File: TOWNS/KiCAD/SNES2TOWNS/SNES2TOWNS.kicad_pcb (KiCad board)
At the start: 2 copper layers, 64.8 x 50.8 mm, 16 parts, among them J1 DE9_Receptacle, J6 SNES_CONTROLLER, J8 ArduinoNANOP1_P15, J9 ArduinoNANOP16_P30, SW1 PCM13SMTR, U1 74HC157, U2 74HC157

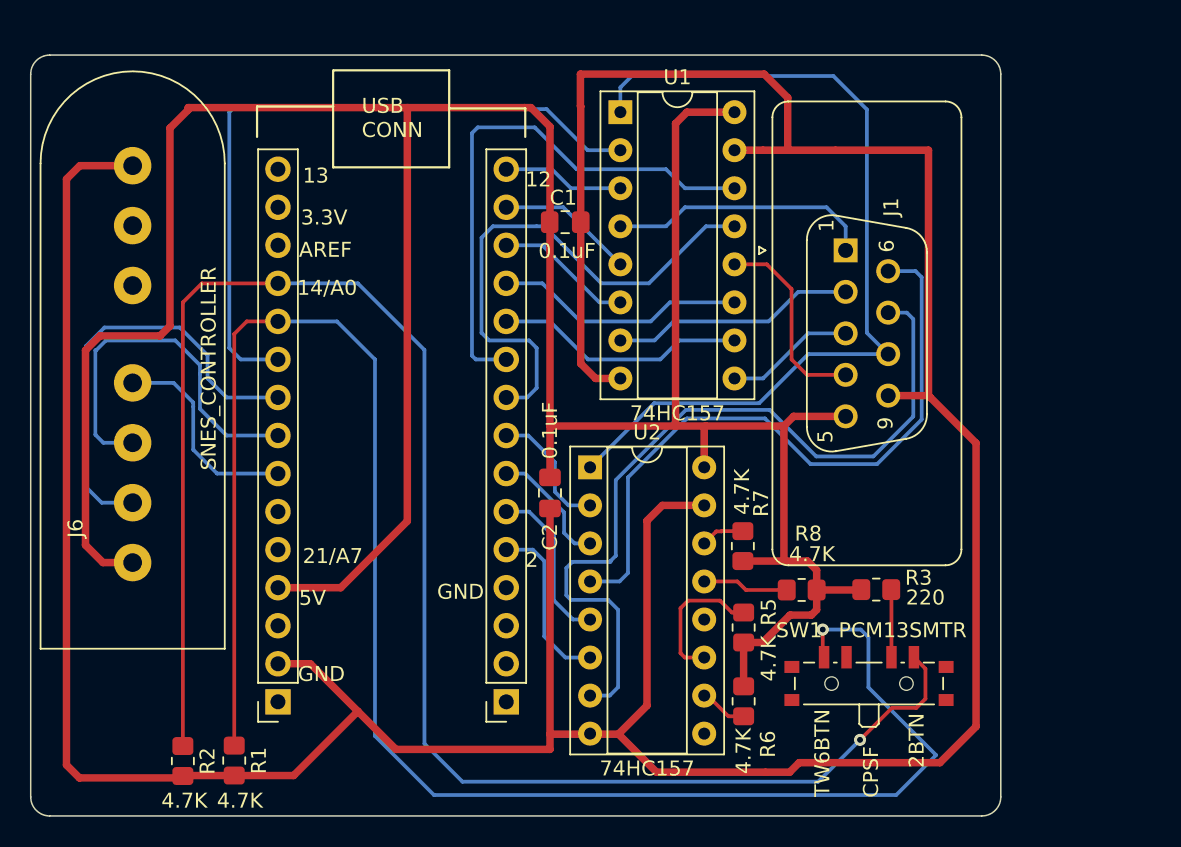
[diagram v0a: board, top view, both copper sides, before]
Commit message: Updating PCB
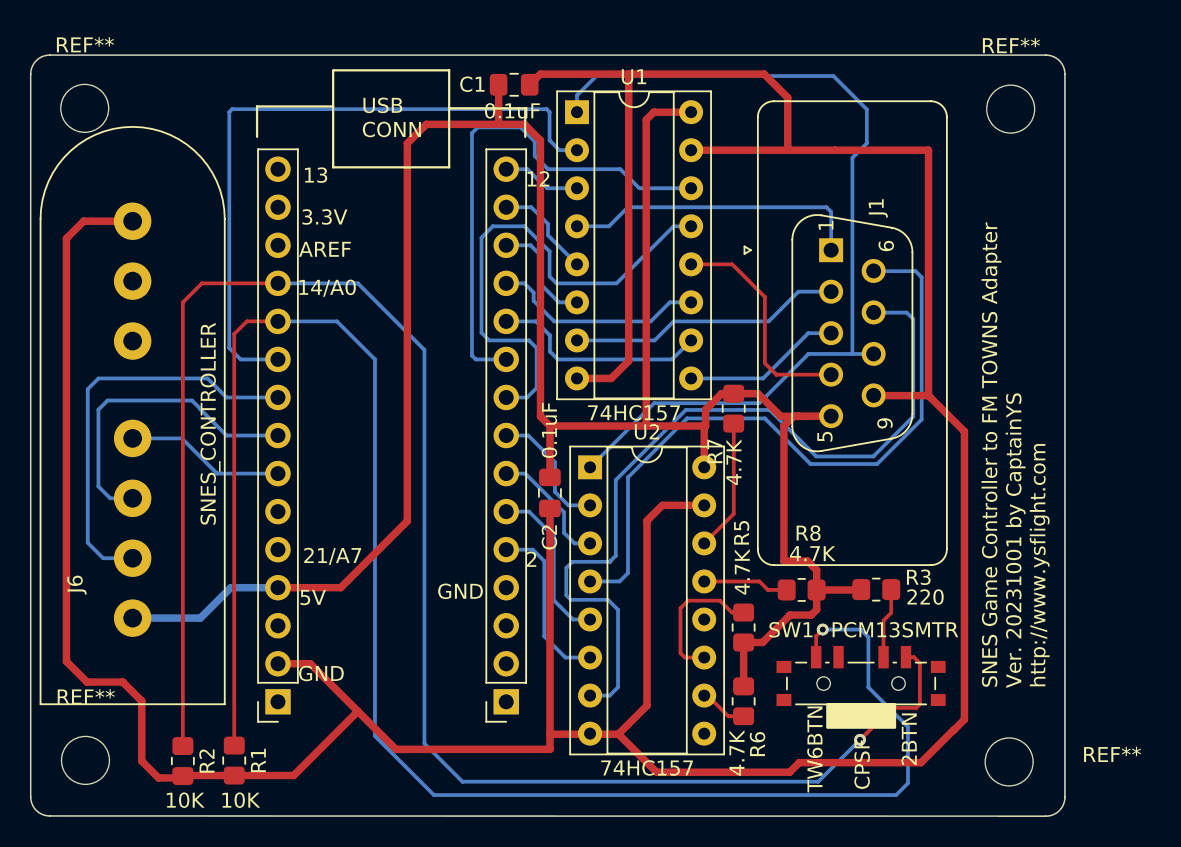
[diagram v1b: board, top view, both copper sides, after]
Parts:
- added REF**: 2.85mm, MountingHole:MountingHole_3.2mm_M3, F.Cu at (109.1, 110.6)
- added REF**: 2.85mm, MountingHole:MountingHole_3.2mm_M3, F.Cu at (109.0, 67.1)
- added REF**: 2.85mm, MountingHole:MountingHole_3.2mm_M3, F.Cu at (170.8, 67.1)
- added REF**: 2.85mm, MountingHole:MountingHole_3.2mm_M3, F.Cu at (170.7, 110.7)
- R1, R2: value 4.7K -> 10K
- moved C1 9.79 mm to (137.7, 65.5)
- moved R7 9.20 mm to (152.3, 87.1), turned to -90 degrees
- moved J6 3.71 mm to (112.2, 101.1)
- moved U1 2.90 mm to (141.9, 67.3)
- moved J1 0.97 mm to (158.9, 76.5)
- moved SW1 0.53 mm to (160.9, 105.1)
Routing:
- net +5V: track 200.0 -> 155.9 mm
- net Net-(U2-I0d): track 2.92 -> 8.81 mm
- net /LATCH: track 25.2 -> 21.0 mm
- net /DATA: track 14.1 -> 10.7 mm
- net /OUT_P1B: track 8.15 -> 5.25 mm
- net /OUT_P3A: track 16.8 -> 14.2 mm
- net /OUT_P1: track 17.7 -> 20.2 mm
- net /OUT_P2A: track 9.20 -> 6.75 mm
- net /OUT_P4A: track 36.6 -> 34.3 mm
- net /OUT_P3B: track 16.8 -> 14.5 mm
- net /CLOCK: track 29.1 -> 27.2 mm
- net /OUT_P3: track 8.67 -> 10.6 mm
- net /OUT_P2: track 16.4 -> 18.3 mm
- net /OUT_P4B: track 35.8 -> 33.9 mm
- net /OUT_P2B: track 9.27 -> 7.43 mm
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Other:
- board size 64.8 x 50.8 mm -> 69.1 x 50.8 mm
- board text added: "SNES Game Controller to FM TOWNS Adapter Ver. 20231001 by CaptainYS http://www.ysflight.com"
- board text removed: "SNES Game Controller to FM TOWNS Adapter Ver. 20230910 by CaptainYS http://www.ysflight.com"
